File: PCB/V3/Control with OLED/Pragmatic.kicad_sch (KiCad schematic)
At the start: 5 parts, among them J1 L, J2 R, J3 OLED, SW1 SW_Push, U1 ProMicro

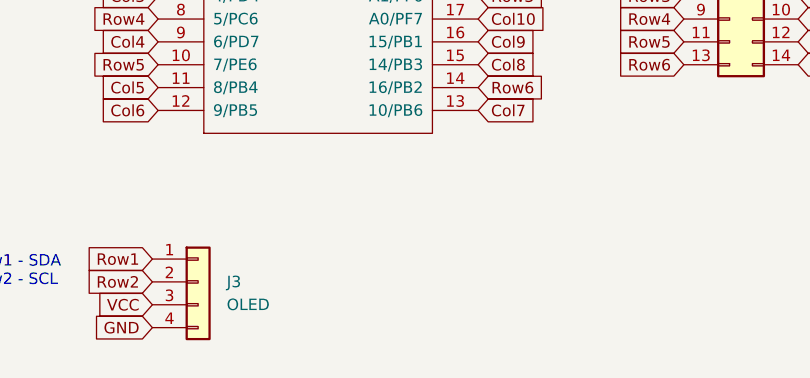
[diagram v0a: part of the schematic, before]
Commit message: prepare for manufacture
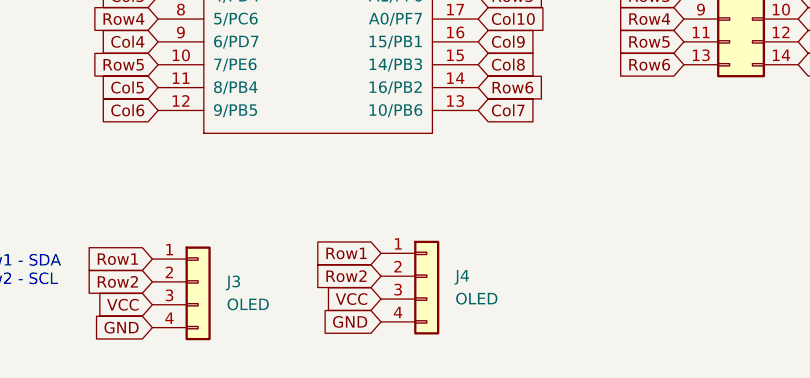
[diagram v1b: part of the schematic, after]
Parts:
- added J4: OLED, Keyboard_JSA:SSD1306_OLED-0.91-128x32, symbol Connector_Generic:Conn_01x04
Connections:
- net +5V: now also J4.3 (Pin_3)
- net GND: now also J4.4 (Pin_4)
- net Row1: now also J4.1 (Pin_1)
- net Row2: now also J4.2 (Pin_2)
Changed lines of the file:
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@@
+    )
+  )
+  (global_label "GND" (shape input) (at 146.685 135.255 180) (fields_autoplaced)
+    (effects (font (size 1.27 1.27)) (justify right))
+    (property "Intersheet References" "${INTERSHEET_REFS}" (id 0) (at 24.765 46.355 0)
+      (effects (font (size 1.27 1.27)) hide)
     )
   )
@@
     )
   )
+  (global_label "Row1" (shape input) (at 146.685 127.635 180) (fields_autoplaced)
+    (effects (font (size 1.27 1.27)) (justify right))
+    (property "Intersheet References" "${INTERSHEET_REFS}" (id 0) (at 139.4018 127.5556 0)
+      (effects (font (size 1.27 1.27)) (justify right) hide)
+    )
+  )
   (global_label "Col1" (shape input) (at 193.04 68.58 0) (fields_autoplaced)
     (effects (font (size 1.27 1.27)) (justify left))
@@
     (effects (font (size 1.27 1.27)) (justify right))
     (property "Intersheet References" "${INTERSHEET_REFS}" (id 0) (at 283.21 172.72 0)
+      (effects (font (size 1.27 1.27)) hide)
+    )
+  )
+  (global_label "VCC" (shape input) (at 146.685 132.715 180) (fields_autoplaced)
+    (effects (font (size 1.27 1.27)) (justify right))
+    (property "Intersheet References" "${INTERSHEET_REFS}" (id 0) (at 304.165 224.155 0)
       (effects (font (size 1.27 1.27)) hide)
     )
@@
     (property "Intersheet References" "${INTERSHEET_REFS}" (id 0) (at 0 -5.08 0)
       (effects (font (size 1.27 1.27)) hide)
+    )
+  )
+  (global_label "Row2" (shape input) (at 146.685 130.175 180) (fields_autoplaced)
+    (effects (font (size 1.27 1.27)) (justify right))
+    (property "Intersheet References" "${INTERSHEET_REFS}" (id 0) (at 139.4018 130.0956 0)
+      (effects (font (size 1.27 1.27)) (justify right) hide)
     )
   )
@@
     (pin "9")
   )
+  (symbol (lib_id "Connector_Generic:Conn_01x04") (at 151.765 130.175 0) (unit 1)
+    (in_bom yes) (on_board yes) (fields_autoplaced)
+    (property "Reference" "J4" (id 0) (at 154.94 130.1749 0)
+      (effects (font (size 1.27 1.27)) (justify left))
+    )
+    (property "Value" "OLED" (id 1) (at 154.94 132.7149 0)
+      (effects (font (size 1.27 1.27)) (justify left))
+    )
+    (property "Footprint" "Keyboard_JSA:SSD1306_OLED-0.91-128x32" (id 2) (at 151.765 130.175 0)
+      (effects (font (size 1.27 1.27)) hide)
+    )
+    (property "Datasheet" "~" (id 3) (at 151.765 130.175 0)
+      (effects (font (size 1.27 1.27)) hide)
+    )
+    (pin "1")
+    (pin "2")
+    (pin "3")
+    (pin "4")
+  )
   (sheet_instances
     (path "/" (page "1"))
@@
       (reference "J3") (unit 1) (value "OLED") (footprint "Keyboard_JSA:SSD1306_OLED-0.91-128x32")
     )
+    (path "/da7c65e8-e6da-4149-8267-8af15cb46e4c"
+      (reference "J4") (unit 1) (value "OLED") (footprint "Keyboard_JSA:SSD1306_OLED-0.91-128x32")
+    )
     (path "/00000000-0000-0000-0000-000061879342"

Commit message: reversed pro micro
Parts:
- U1: footprint Keyboard_JSA:ArduinoProMicro -> Keyboard_JSA:ProMicro Reversed
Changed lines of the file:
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@@
       (effects (font (size 1.524 1.524)))
     )
-    (property "Footprint" "Keyboard_JSA:ArduinoProMicro" (id 2) (at 166.37 161.29 90)
+    (property "Footprint" "Keyboard_JSA:ProMicro Reversed" (id 2) (at 166.37 161.29 90)
       (effects (font (size 1.524 1.524)) hide)
     )
@@
     )
     (path "/c77559f1-9310-438e-bb42-9cac3de0d116"
-      (reference "U1") (unit 1) (value "ProMicro") (footprint "Keyboard_JSA:ArduinoProMicro")
+      (reference "U1") (unit 1) (value "ProMicro") (footprint "Keyboard_JSA:ProMicro Reversed")
     )
   )
